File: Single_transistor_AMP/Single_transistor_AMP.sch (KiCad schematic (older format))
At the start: 14 parts, among them J1 AudioJack2_Ground, J2 32V, J3 Signal out, Q1 BC546, Q3 TIP140

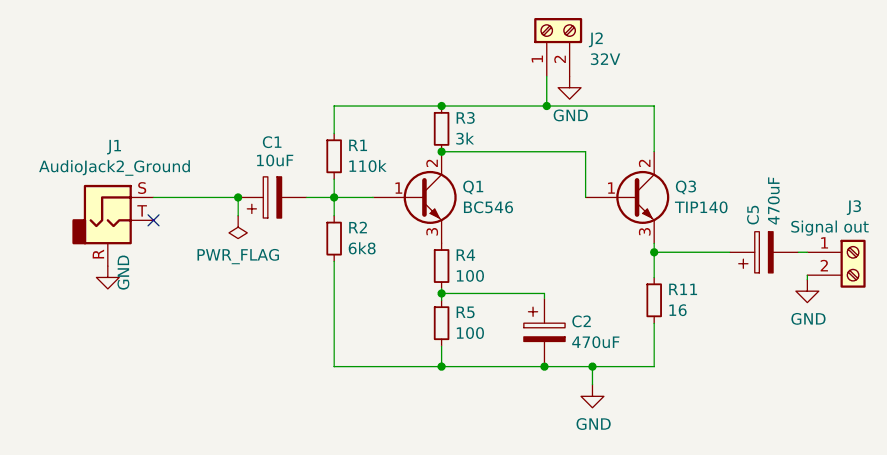
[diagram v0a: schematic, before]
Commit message: 8 nodarbības MD
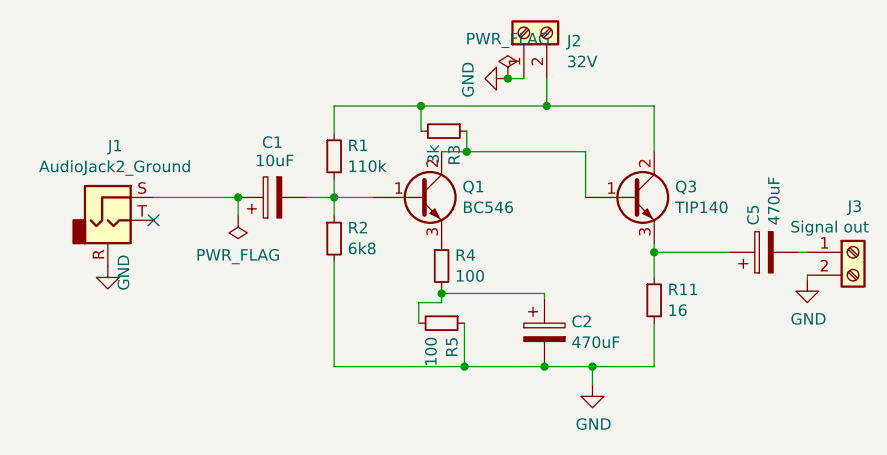
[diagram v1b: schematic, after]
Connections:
- net GND: now also J2.1 (Pin_1), R5.1; no longer J2.2 (Pin_2), R5.2
- net at Q1.2 (C), Q3.1 (B): now also R3.1; no longer R3.2
- net at Q3.2 (C), R1.1: now also J2.2 (Pin_2), R3.2; no longer J2.1 (Pin_1), R3.1
- net at C2.1, R4.2: now also R5.2; no longer R5.1
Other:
- moved on the sheet: J2
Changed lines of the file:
@@
 	0    -1   -1   0
-$EndComp
-$Comp
-L power:GND #PWR01
-U 1 1 5F8B5E0C
-P 5090 3110
-F 0 "#PWR01" H 5090 2860 50  0001 C CNN
-F 1 "GND" H 5095 2937 50  0000 C CNN
-F 2 "" H 5090 3110 50  0001 C CNN
-F 3 "" H 5090 3110 50  0001 C CNN
-	1    5090 3110
-	1    0    0    -1
 $EndComp
 Wire Wire Line
@@
 	4420 2990 4420 3100
 NoConn ~ 2230 2850
-$Comp
-L Connector:Screw_Terminal_01x02 J3
-U 1 1 5F8C6ECE
-P 5290 2990
-F 0 "J3" H 5330 3190 50  0000 R CNN
-F 1 "Signal out" H 5360 3100 50  0000 R CNN
-F 2 "Connector:JWT_A3963_1x02_P3.96mm_Vertical" H 5290 2990 50  0001 C CNN
-F 3 "~" H 5290 2990 50  0001 C CNN
-	1    5290 2990
-	1    0    0    -1
-$EndComp
 Wire Wire Line
 	2600 2750 2230 2750
 Connection ~ 2600 2750
-Wire Wire Line
-	3490 3170 3490 3200
 Wire Wire Line
 	3940 3170 3490 3170
@@
 Wire Wire Line
 	4150 3570 4150 3490
-Wire Wire Line
-	3950 2220 3950 2350
 $Comp
 L power:GND #PWR0104
 U 1 1 5F8A30A1
-P 4050 2220
-F 0 "#PWR0104" H 4050 1970 50  0001 C CNN
-F 1 "GND" H 4055 2047 50  0000 C CNN
-F 2 "" H 4050 2220 50  0001 C CNN
-F 3 "" H 4050 2220 50  0001 C CNN
-	1    4050 2220
-	1    0    0    -1
+P 3780 2230
+F 0 "#PWR0104" H 3780 1980 50  0001 C CNN
+F 1 "GND" H 3785 2057 50  0000 C CNN
+F 2 "" H 3780 2230 50  0001 C CNN
+F 3 "" H 3780 2230 50  0001 C CNN
+	1    3780 2230
+	0    1    1    0
 $EndComp
 $Comp
 L Connector:Screw_Terminal_01x02 J2
 U 1 1 5F89E0FF
-P 3950 2020
-F 0 "J2" V 3914 1832 50  0000 R CNN
-F 1 "32V" V 3823 1832 50  0000 R CNN
-F 2 "Connector:JWT_A3963_1x02_P3.96mm_Vertical" H 3950 2020 50  0001 C CNN
-F 3 "~" H 3950 2020 50  0001 C CNN
-	1    3950 2020
+P 3850 2030
+F 0 "J2" V 3814 1842 50  0000 R CNN
+F 1 "32V" V 3723 1842 50  0000 R CNN
+F 2 "Connector:JWT_A3963_1x02_P3.96mm_Vertical" H 3850 2030 50  0001 C CNN
+F 3 "~" H 3850 2030 50  0001 C CNN
+	1    3850 2030
 	0    -1   -1   0
 $EndComp
@@
 Wire Wire Line
 	4120 2550 4120 2750
-Wire Wire Line
-	3490 2550 4120 2550
-Wire Wire Line
-	3490 2350 3950 2350
-Wire Wire Line
-	3490 2350 3020 2350
-Connection ~ 3490 2350
 $Comp
 L Device:R_Small R3
 U 1 1 5F8829A4
-P 3490 2450
-F 0 "R3" H 3549 2496 50  0000 L CNN
-F 1 "3k" H 3549 2405 50  0000 L CNN
-F 2 "Resistor_SMD:R_0603_1608Metric" H 3490 2450 50  0001 C CNN
-F 3 "http://www.farnell.com/datasheets/2339608.pdf" H 3490 2450 50  0001 C CNN
-F 4 "https://lv.farnell.com/vishay/crcw04022k70fkedhp/res-2k7-1-0-2w-0402-thick-film/dp/1738855RL?st=2.7kohm" H 3490 2450 50  0001 C CNN "Farnell"
-	1    3490 2450
-	1    0    0    -1
-$EndComp
-Wire Wire Line
-	3020 3490 3490 3490
-Connection ~ 3490 3490
-Wire Wire Line
-	3490 3490 3490 3400
+P 3500 2460
+F 0 "R3" H 3559 2506 50  0000 L CNN
+F 1 "3k" H 3559 2415 50  0000 L CNN
+F 2 "Resistor_SMD:R_0603_1608Metric" H 3500 2460 50  0001 C CNN
+F 3 "http://www.farnell.com/datasheets/2339608.pdf" H 3500 2460 50  0001 C CNN
+F 4 "https://lv.farnell.com/vishay/crcw04022k70fkedhp/res-2k7-1-0-2w-0402-thick-film/dp/1738855RL?st=2.7kohm" H 3500 2460 50  0001 C CNN "Farnell"
+	1    3500 2460
+	0    1    1    0
+$EndComp
 Wire Wire Line
 	3940 3170 3940 3190
 Wire Wire Line
 	3940 3490 4150 3490
-Wire Wire Line
-	3490 3490 3940 3490
 Connection ~ 3940 3490
 $Comp
@@
 F 4 "https://lv.farnell.com/vishay/crcw0805120rfkea/res-120r-1-0-125w-0805-thick-film/dp/1652914?st=120%20ohm" H 3490 3300 50  0001 C CNN "Farnell"
 	1    3490 3300
-	1    0    0    -1
-$EndComp
-Connection ~ 3490 2550
+	0    1    1    0
+$EndComp
 $Comp
 L Device:Q_NPN_BCE Q1
@@
 $EndComp
 Wire Wire Line
-	3950 2350 4420 2350
-Connection ~ 3950 2350
-Wire Wire Line
 	4420 2350 4420 2550
 Wire Wire Line
@@
 Wire Wire Line
 	5090 2990 5050 2990
-Wire Wire Line
-	5090 3090 5090 3110
 $Comp
 L Connector:AudioJack2_Ground J1
@@
 	1    0    0    -1
 $EndComp
+Wire Wire Line
+	5090 3090 5090 3110
+$Comp
+L power:GND #PWR01
+U 1 1 5F8B5E0C
+P 5090 3110
+F 0 "#PWR01" H 5090 2860 50  0001 C CNN
+F 1 "GND" H 5095 2937 50  0000 C CNN
+F 2 "" H 5090 3110 50  0001 C CNN
+F 3 "" H 5090 3110 50  0001 C CNN
+	1    5090 3110
+	1    0    0    -1
+$EndComp
+$Comp
+L Connector:Screw_Terminal_01x02 J3
+U 1 1 5F8C6ECE
+P 5290 2990
+F 0 "J3" H 5330 3190 50  0000 R CNN
+F 1 "Signal out" H 5360 3100 50  0000 R CNN
+F 2 "Connector:JWT_A3963_1x02_P3.96mm_Vertical" H 5290 2990 50  0001 C CNN
+F 3 "~" H 5290 2990 50  0001 C CNN
+	1    5290 2990
+	1    0    0    -1
+$EndComp
+Wire Wire Line
+	3950 2230 3950 2350
+Connection ~ 3950 2350
+Wire Wire Line
+	3950 2350 4420 2350
+$Comp
+L power:PWR_FLAG #FLG?
+U 1 1 5FC779AA
+P 3780 2230
+F 0 "#FLG?" H 3780 2305 50  0001 C CNN
+F 1 "PWR_FLAG" H 3780 2403 50  0000 C CNN
+F 2 "" H 3780 2230 50  0001 C CNN
+F 3 "~" H 3780 2230 50  0001 C CNN
+	1    3780 2230
+	1    0    0    -1
+$EndComp
+Wire Wire Line
+	3850 2230 3780 2230
+Connection ~ 3780 2230
+Wire Wire Line
+	3400 2350 3400 2460
+Wire Wire Line
+	3020 2350 3400 2350
+Connection ~ 3400 2350
+Wire Wire Line
+	3600 2460 3600 2550
+Wire Wire Line
+	3490 2550 3600 2550
+Wire Wire Line
+	3400 2350 3950 2350
+Connection ~ 3600 2550
+Wire Wire Line
+	3600 2550 4120 2550
+Wire Wire Line
+	3490 3210 3390 3210
+Wire Wire Line
+	3390 3210 3390 3300
+Wire Wire Line
+	3490 3170 3490 3210
+Wire Wire Line
+	3590 3300 3590 3490
+Connection ~ 3590 3490
+Wire Wire Line
+	3590 3490 3940 3490
+Wire Wire Line
+	3020 3490 3590 3490
 $EndSCHEMATC
